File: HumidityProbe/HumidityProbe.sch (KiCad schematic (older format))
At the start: 10 parts

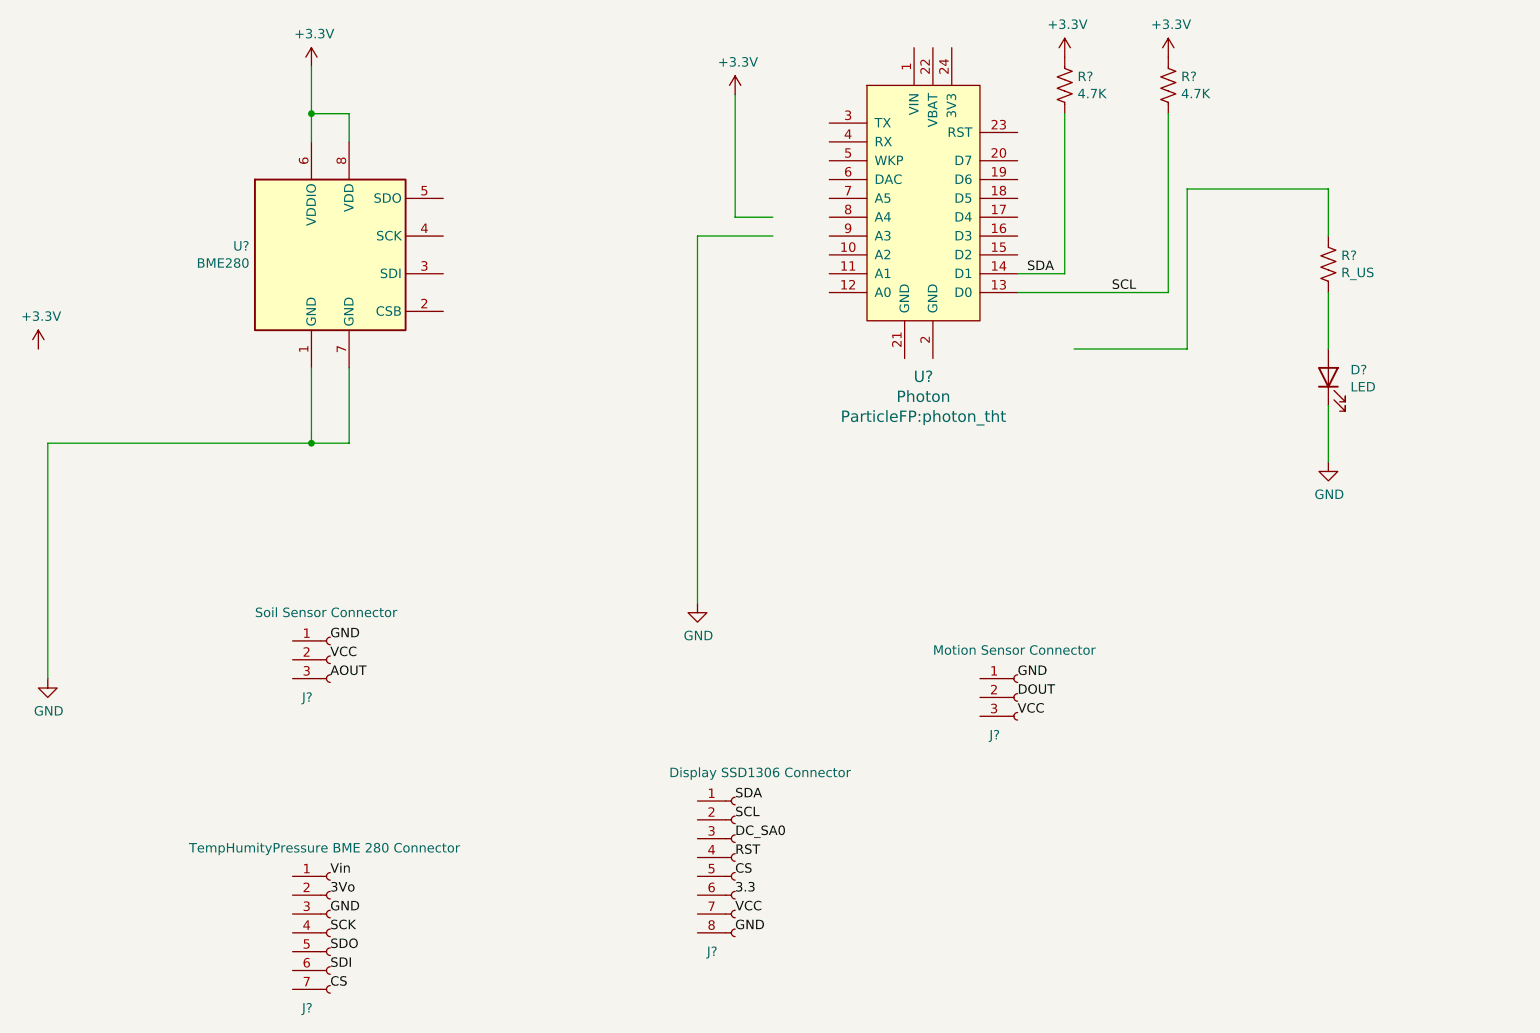
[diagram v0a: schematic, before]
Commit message: some connections
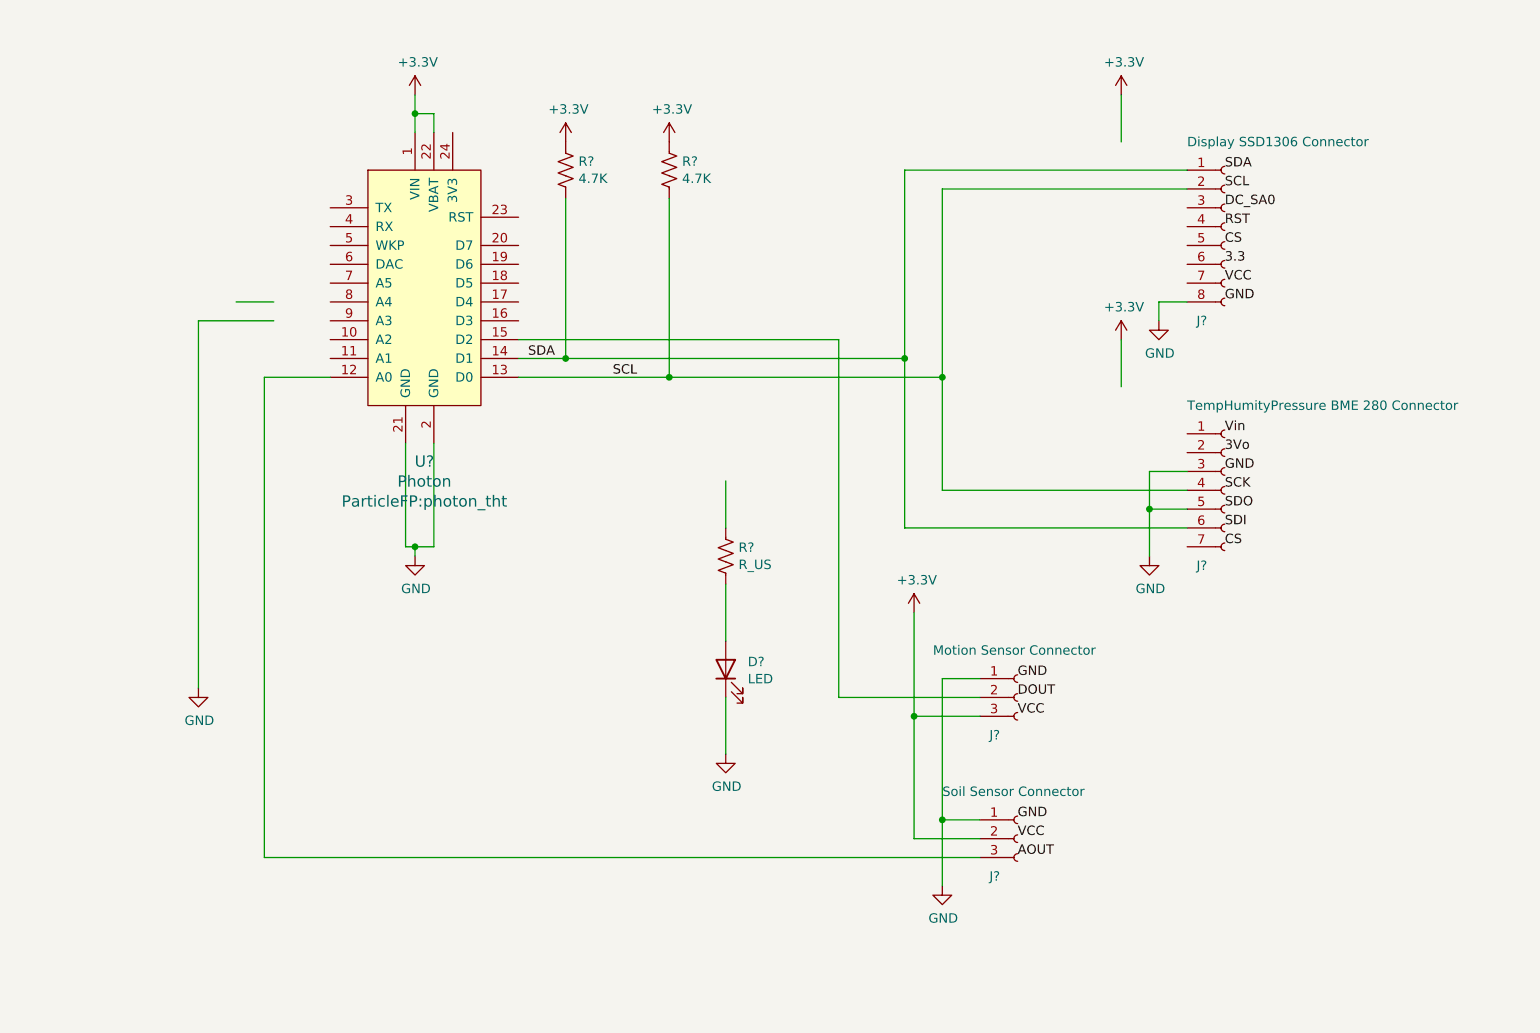
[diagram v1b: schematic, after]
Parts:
- removed U?: BME280, Package_LGA:Bosch_LGA-8_2.5x2.5mm_P0.65mm_ClockwisePinNumbering, symbol Sensor:BME280
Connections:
- wire segments 23 -> 51
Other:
- moved on the sheet: D?, J?, R?, U?
